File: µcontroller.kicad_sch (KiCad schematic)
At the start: 18 parts, among them U1 stm32G4, Y2 8Mhz

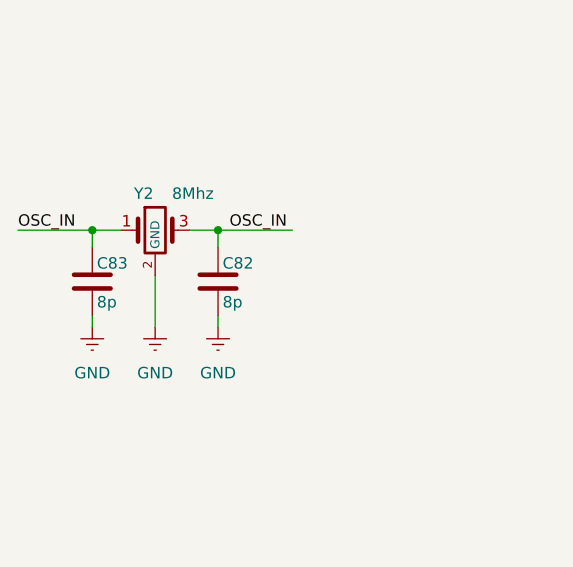
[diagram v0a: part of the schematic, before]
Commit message: al de main blokken bij elkaar gezet op juiste plaats
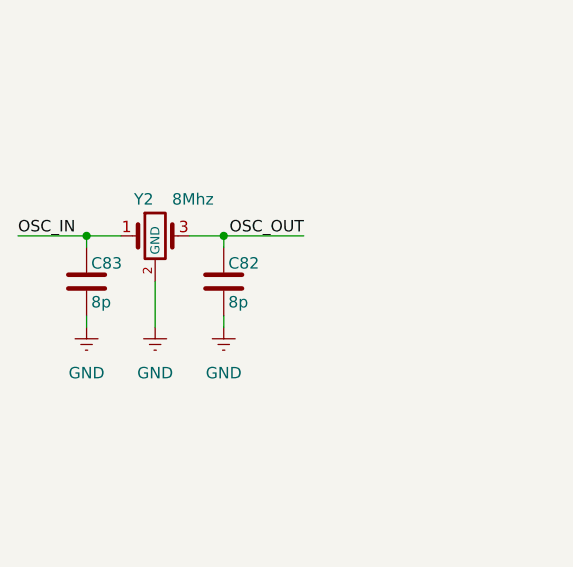
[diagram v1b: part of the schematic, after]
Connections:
- net GND: now also Y2.4 (GND)
- net OSC_IN: no longer C82.1, Y2.3
- net OSC_OUT: now also C82.1, Y2.3
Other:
- moved on the sheet: C82, C83, Y2
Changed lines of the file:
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@@
 	)
 	(junction
-		(at 67.945 99.695)
+		(at 68.58 100.33)
 		(diameter 0)
 		(color 0 0 0 0)
@@
 	)
 	(junction
-		(at 53.975 99.695)
+		(at 53.34 100.33)
 		(diameter 0)
 		(color 0 0 0 0)
@@
 	(wire
 		(pts
-			(xy 64.77 99.695) (xy 67.945 99.695)
+			(xy 64.77 100.33) (xy 77.47 100.33)
 		)
 		(stroke
@@
 	(wire
 		(pts
-			(xy 53.975 99.695) (xy 57.15 99.695)
-		)
-		(stroke
-			(width 0)
-			(type default)
-		)
-	)
-	(wire
-		(pts
 			(xy 154.94 85.09) (xy 158.75 85.09)
 		)
@@
 	(wire
 		(pts
-			(xy 53.975 99.695) (xy 53.975 101.6)
+			(xy 53.34 100.33) (xy 53.34 101.6)
 		)
 		(stroke
@@
 	(wire
 		(pts
+			(xy 60.96 105.41) (xy 60.96 110.49)
+		)
+		(stroke
+			(width 0)
+			(type default)
+		)
+	)
+	(wire
+		(pts
 			(xy 188.595 35.56) (xy 194.945 35.56)
 		)
@@
 	(wire
 		(pts
-			(xy 45.72 99.695) (xy 53.975 99.695)
+			(xy 45.72 100.33) (xy 57.15 100.33)
 		)
 		(stroke
@@
 	(wire
 		(pts
-			(xy 67.945 109.22) (xy 67.945 110.49)
+			(xy 68.58 109.22) (xy 68.58 110.49)
 		)
 		(stroke
@@
 	(wire
 		(pts
-			(xy 67.945 99.695) (xy 67.945 101.6)
+			(xy 68.58 100.33) (xy 68.58 101.6)
 		)
 		(stroke
@@
 	(wire
 		(pts
-			(xy 53.975 109.22) (xy 53.975 110.49)
+			(xy 53.34 109.22) (xy 53.34 110.49)
 		)
 		(stroke
@@
 	(wire
 		(pts
-			(xy 60.96 104.775) (xy 60.96 110.49)
-		)
-		(stroke
-			(width 0)
-			(type default)
-		)
-	)
-	(wire
-		(pts
 			(xy 134.62 186.69) (xy 134.62 189.23)
 		)
@@
 	(wire
 		(pts
-			(xy 67.945 99.695) (xy 76.2 99.695)
-		)
-		(stroke
-			(width 0)
-			(type default)
-		)
-	)
-	(wire
-		(pts
 			(xy 127 35.56) (xy 129.54 35.56)
 		)
@@
 		)
 	)
-	(label "OSC_IN"
-		(at 69.215 99.695 0)
+	(label "OSC_OUT"
+		(at 69.215 100.33 0)
 		(effects
 			(font
@@
 	)
 	(label "OSC_IN"
-		(at 45.72 99.695 0)
+		(at 45.72 100.33 0)
 		(effects
 			(font
@@
 	(symbol
 		(lib_id "Device:C")
-		(at 67.945 105.41 0)
+		(at 68.58 105.41 0)
 		(unit 1)
 		(body_style 1)
@@
 		(dnp no)
 		(property "Reference" "C82"
-			(at 68.453 103.378 0)
+			(at 69.088 103.378 0)
 			(show_name no)
 			(do_not_autoplace no)
@@
 		)
 		(property "Value" "8p"
-			(at 68.453 107.696 0)
+			(at 69.088 107.696 0)
 			(show_name no)
 			(do_not_autoplace no)
@@
 		)
 		(property "Footprint" "Capacitor_SMD:C_0603_1608Metric"
-			(at 68.9102 109.22 0)
+			(at 69.5452 109.22 0)
 			(hide yes)
 			(show_name no)
@@
 		)
 		(property "Datasheet" ""
-			(at 67.945 105.41 0)
+			(at 68.58 105.41 0)
 			(hide yes)
 			(show_name no)
@@
 		)
 		(property "Description" "Unpolarized capacitor"
-			(at 67.945 105.41 0)
+			(at 68.58 105.41 0)
 			(hide yes)
 			(show_name no)
@@
 	(symbol
 		(lib_id "Device:C")
-		(at 53.975 105.41 0)
+		(at 53.34 105.41 0)
 		(unit 1)
 		(body_style 1)
@@
 		(dnp no)
 		(property "Reference" "C83"
-			(at 54.483 103.378 0)
+			(at 53.848 103.378 0)
 			(show_name no)
 			(do_not_autoplace no)
@@
 		)
 		(property "Value" "8p"
-			(at 54.483 107.696 0)
+			(at 53.848 107.696 0)
 			(show_name no)
 			(do_not_autoplace no)
@@
 		)
 		(property "Footprint" "Capacitor_SMD:C_0603_1608Metric"
-			(at 54.9402 109.22 0)
+			(at 54.3052 109.22 0)
 			(hide yes)
 			(show_name no)
@@
 		)
 		(property "Datasheet" ""
-			(at 53.975 105.41 0)
+			(at 53.34 105.41 0)
 			(hide yes)
 			(show_name no)
@@
 		)
 		(property "Description" "Unpolarized capacitor"
-			(at 53.975 105.41 0)
+			(at 53.34 105.41 0)
 			(hide yes)
 			(show_name no)
@@
 	(symbol
 		(lib_id "Schemasymbolen_samen:25Mhz_crystal")
-		(at 57.15 98.425 0)
+		(at 57.15 99.06 0)
 		(unit 1)
 		(body_style 1)
@@
 		(dnp no)
 		(property "Reference" "Y2"
-			(at 59.69 95.631 0)
+			(at 59.69 96.266 0)
 			(show_name no)
 			(do_not_autoplace no)
@@
 		)
 		(property "Value" "8Mhz"
-			(at 65.151 95.631 0)
+			(at 65.151 96.266 0)
 			(show_name no)
 			(do_not_autoplace no)
@@
 		)
 		(property "Footprint" "Footprintsymbolen_samen:25Mhz crystal 8pF"
-			(at 52.578 88.011 0)
+			(at 52.578 88.646 0)
 			(hide yes)
 			(show_name no)
@@
 		)
 		(property "Datasheet" "https://www.mouser.be/datasheet/3/1460/1/LFXTAL085880.pdf"
-			(at 73.152 92.837 0)
+			(at 73.152 93.472 0)
 			(hide yes)
 			(show_name no)
@@
 		)
 		(property "Description" "LFXTAL085880"
-			(at 57.15 98.425 0)
+			(at 48.768 95.504 0)
 			(hide yes)
 			(show_name no)
@@
 	(symbol
 		(lib_id "power:GNDREF")
-		(at 53.975 110.49 0)
+		(at 53.34 110.49 0)
 		(unit 1)
 		(body_style 1)
@@
 		(fields_autoplaced yes)
 		(property "Reference" "#PWR0103"
-			(at 53.975 116.84 0)
+			(at 53.34 116.84 0)
 			(hide yes)
 			(show_name no)
@@
 		)
 		(property "Value" "GND"
-			(at 53.975 115.57 0)
+			(at 53.34 115.57 0)
 			(show_name no)
 			(do_not_autoplace no)
@@
 		)
 		(property "Footprint" ""
-			(at 53.975 110.49 0)
+			(at 53.34 110.49 0)
 			(hide yes)
 			(show_name no)
@@
 		)
 		(property "Datasheet" ""
-			(at 53.975 110.49 0)
+			(at 53.34 110.49 0)
 			(hide yes)
 			(show_name no)
@@
 		)
 		(property "Description" "Power symbol creates a global label with name \"GNDREF\" , reference supply ground"
-			(at 53.975 110.49 0)
+			(at 53.34 110.49 0)
 			(hide yes)
 			(show_name no)
@@
 	(symbol
 		(lib_id "power:GNDREF")
-		(at 67.945 110.49 0)
+		(at 68.58 110.49 0)
 		(unit 1)
 		(body_style 1)
@@
 		(fields_autoplaced yes)
 		(property "Reference" "#PWR0102"
-			(at 67.945 116.84 0)
+			(at 68.58 116.84 0)
 			(hide yes)
 			(show_name no)
@@
 		)
 		(property "Value" "GND"
-			(at 67.945 115.57 0)
+			(at 68.58 115.57 0)
 			(show_name no)
 			(do_not_autoplace no)
@@
 		)
 		(property "Footprint" ""
-			(at 67.945 110.49 0)
+			(at 68.58 110.49 0)
 			(hide yes)
 			(show_name no)
@@
 		)
 		(property "Datasheet" ""
-			(at 67.945 110.49 0)
+			(at 68.58 110.49 0)
 			(hide yes)
 			(show_name no)
@@
 		)
 		(property "Description" "Power symbol creates a global label with name \"GNDREF\" , reference supply ground"
-			(at 67.945 110.49 0)
+			(at 68.58 110.49 0)
 			(hide yes)
 			(show_name no)
